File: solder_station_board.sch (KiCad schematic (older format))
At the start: 41 parts, among them J1 PWR_5_V, J2 INPUT, J3 RT_WELLER, J4 INPUT, J5 VFD_DISPLAY, J6 PWR_15V, J8 SERIAL, P1 ISP, Q1 IRF9540, Q2 2N7002, U4 TLC272, U5 LT1007, U6 ATMEGA168-20AU

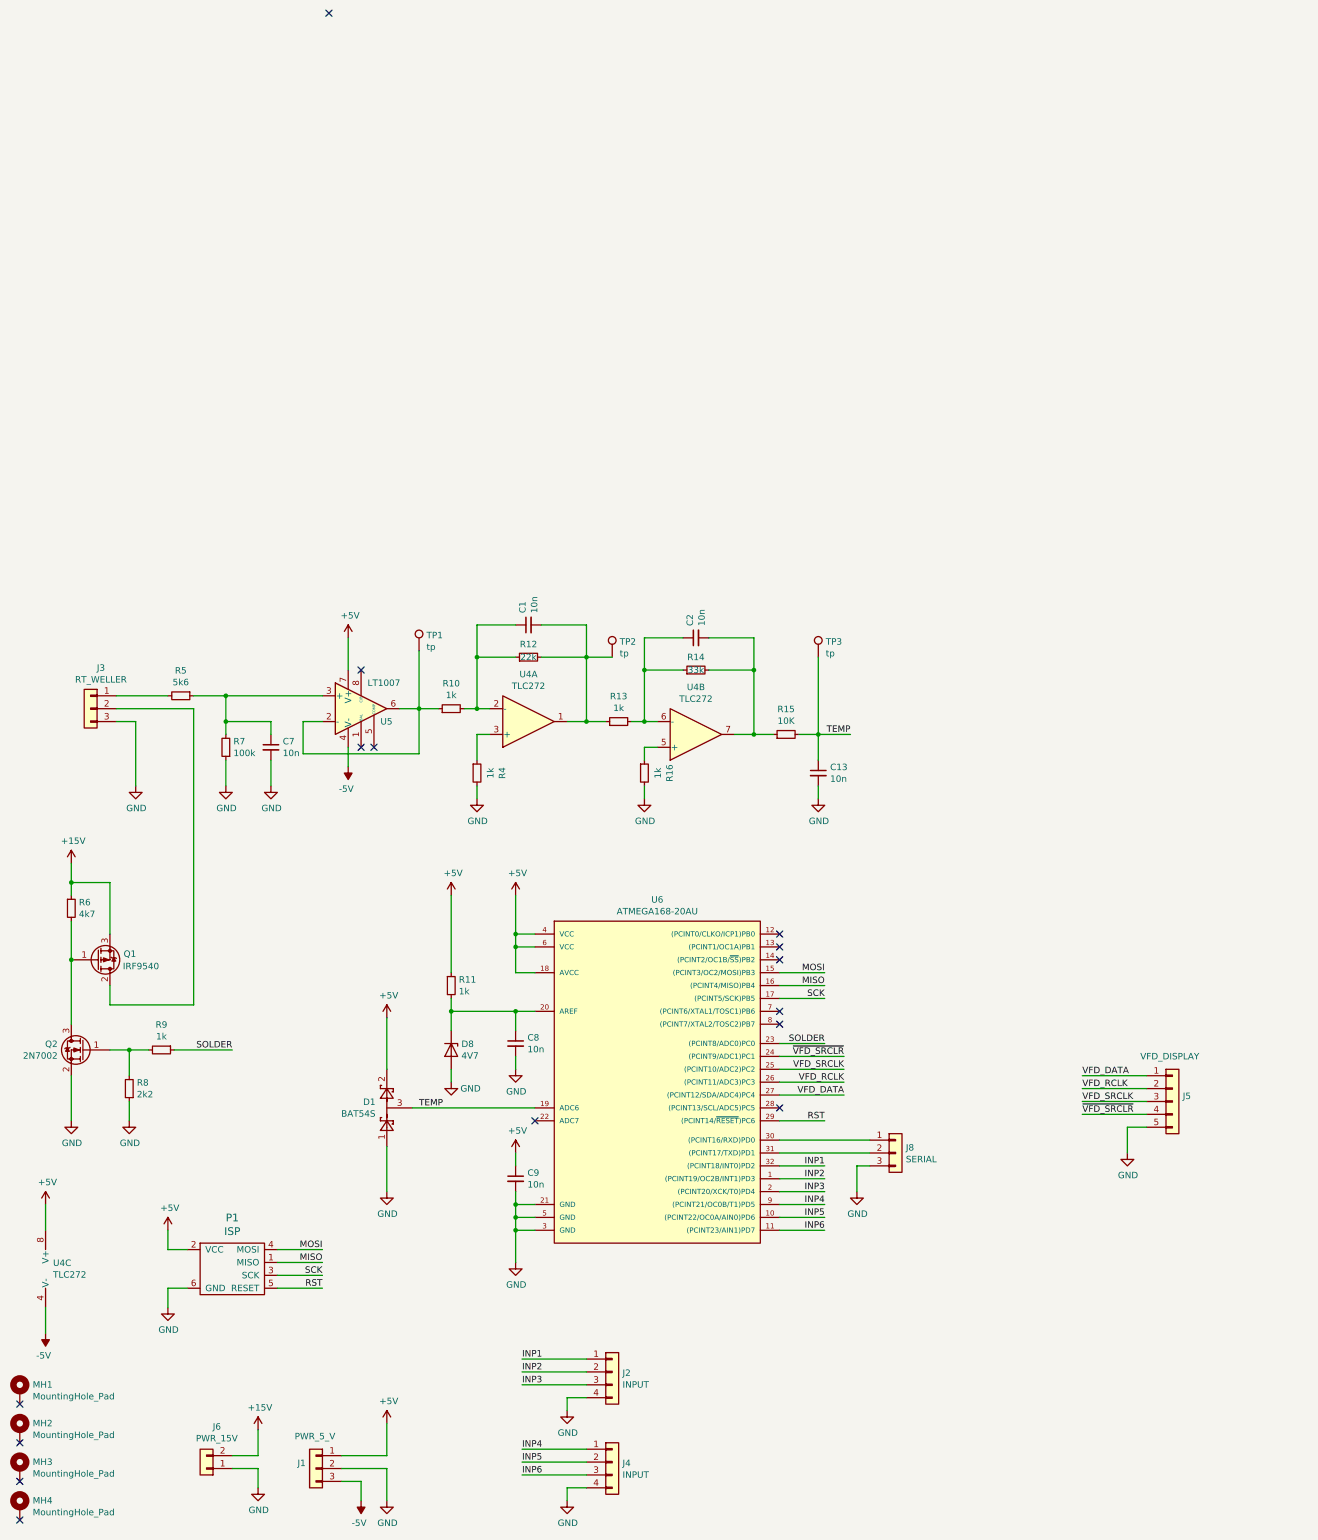
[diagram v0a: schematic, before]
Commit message: small arrangements
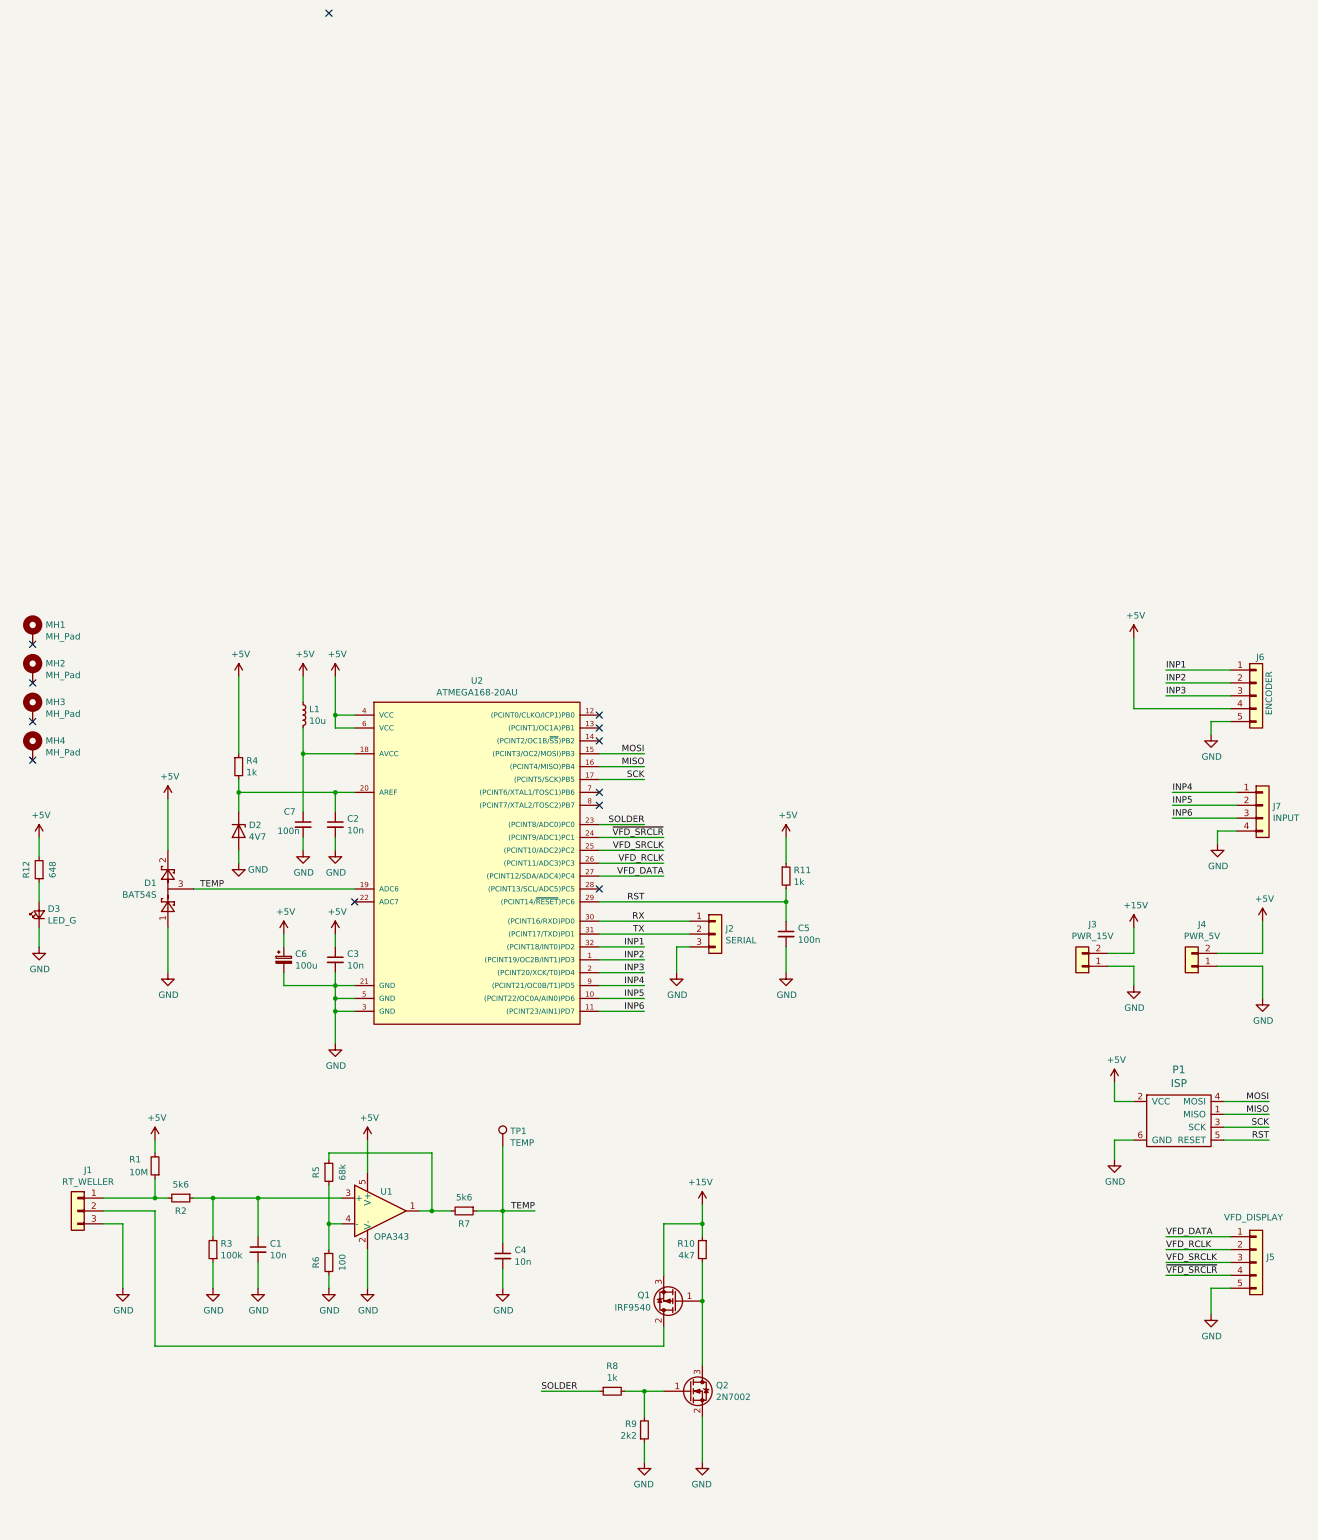
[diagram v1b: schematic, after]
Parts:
- removed C1, C13, C2: 10n, Capacitor_SMD:C_0805_2012Metric_Pad1.15x1.40mm_HandSolder, symbol Device:C_Small
- removed J1: PWR_5_V, Connector_PinSocket_2.54mm:PinSocket_1x03_P2.54mm_Vertical, symbol Connector_Generic:Conn_01x03
- removed J2: INPUT, Connector_PinHeader_2.54mm:PinHeader_1x04_P2.54mm_Vertical, symbol Connector_Generic:Conn_01x04
- removed R13, R16, R4: 1k, Resistor_SMD:R_0805_2012Metric_Pad1.15x1.40mm_HandSolder, symbol Device:R_Small
- removed R14: 33k, Resistor_SMD:R_0805_2012Metric_Pad1.15x1.40mm_HandSolder, symbol Device:R_Small
- removed R15: 10K, Resistor_SMD:R_0805_2012Metric_Pad1.15x1.40mm_HandSolder, symbol Device:R_Small
- removed TP1, TP2, TP3: tp, Connector_Wire:SolderWirePad_1x01_Drill0.8mm, symbol solder_station_board-rescue:TestPoint-Connector
- removed U4: TLC272, Package_SO:SOIC-8_3.9x4.9mm_P1.27mm, symbol Amplifier_Operational:TLC272
- removed U5: LT1007, Package_SO:SOIC-8_3.9x4.9mm_P1.27mm, symbol Amplifier_Operational:LT1012
- added C4: 10n, Capacitor_SMD:C_0805_2012Metric_Pad1.15x1.40mm_HandSolder, symbol Device:C_Small
- added C5, C7: 100n, Capacitor_SMD:C_0805_2012Metric_Pad1.15x1.40mm_HandSolder, symbol Device:C_Small
- added C6: 100u, Capacitor_THT:C_Radial_D8.0mm_H7.0mm_P3.50mm, symbol Device:CP_Small
- added D3: LED_G, LED_THT:LED_D3.0mm, symbol solder_station_board-rescue:LED_Small-custom
- added J4: PWR_5V, Connector_PinHeader_2.54mm:PinHeader_1x02_P2.54mm_Vertical, symbol Connector_Generic:Conn_01x02
- added J6: ENCODER, Connector_PinHeader_2.54mm:PinHeader_1x05_P2.54mm_Vertical, symbol Connector_Generic:Conn_01x05
- added L1: 10u, Inductor_SMD:L_1206_3216Metric_Pad1.42x1.75mm_HandSolder, symbol Device:L_Small
- added R1: 10M, Resistor_SMD:R_0805_2012Metric_Pad1.15x1.40mm_HandSolder, symbol Device:R_Small
- added R11: 1k, Resistor_SMD:R_0805_2012Metric_Pad1.15x1.40mm_HandSolder, symbol Device:R_Small
- added R5: 68k, Resistor_SMD:R_0805_2012Metric_Pad1.15x1.40mm_HandSolder, symbol Device:R_Small
- added R7: 5k6, Resistor_SMD:R_0805_2012Metric_Pad1.15x1.40mm_HandSolder, symbol Device:R_Small
- added TP1: TEMP, TestPoint:TestPoint_Loop_D2.60mm_Drill0.9mm_Beaded, symbol Connector:TestPoint
- added U1: OPA343, Package_TO_SOT_SMD:SOT-23-5, symbol Amplifier_Operational:OPA340NA
- MH1, MH2, MH3, MH4: value MountingHole_Pad -> MH_Pad
- R12: value 22k -> 648
- R6: renamed from R10; value 1k -> 100
- renumbered C7 to C1, C8 to C2, C9 to C3, D8 to D2, J3 to J1, J8 to J2, J6 to J3, J4 to J7, R6 to R10, R5 to R2, R7 to R3, R11 to R4, R9 to R8, R8 to R9, U6 to U2
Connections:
- net +5V: now also R12.2, C6.1, J4.2 (Pin_2), J6.4 (Pin_4), L1.1, R1.2, R11.1, U1.5 (V+); no longer U2.18 (AVCC)
- net GND: now also R6.2, C4.2, C5.2, C6.2, C7.2, D3.1 (K), J4.1 (Pin_1), J6.5 (Pin_5), U1.2 (V-)
- net INP1: now also J6.1 (Pin_1)
- net INP2: now also J6.2 (Pin_2)
- net INP3: now also J6.3 (Pin_3)
- net RST: now also C5.1, R11.2
- net TEMP: now also C4.1, R7.1, TP1.1
- net at J1.1 (Pin_1), R2.2: now also R1.1
- net at C1.1, R2.1, R3.2: now also U1.3 (+)
- net at R12.1: now also D3.2 (A); no longer R6.2
- net at R6.1: now also R5.2, U1.4 (-)
- net RX: now reaches J2.1 (Pin_1), U2.30 ((PCINT16/RXD)PD0)
- net TX: now reaches J2.2 (Pin_2), U2.31 ((PCINT17/TXD)PD1)
- new net: C7.1, L1.2, U2.18 (AVCC)
- new net: R5.1, R7.2, U1.1
- no-connect marks 15 -> 12
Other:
- moved on the sheet: C1, C2, C3, D1, D2, J1, J2, J3, J5, J7, MH1, MH2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
